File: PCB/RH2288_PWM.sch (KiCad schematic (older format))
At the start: 10 parts, among them J1 Conn_01x01, J2 AVR_ICSP, J3 Conn_FANs, J4 Conn_RH2288_V2, J5 UART, U1 78L05_SOT23, U2 ATmega328P-MMH

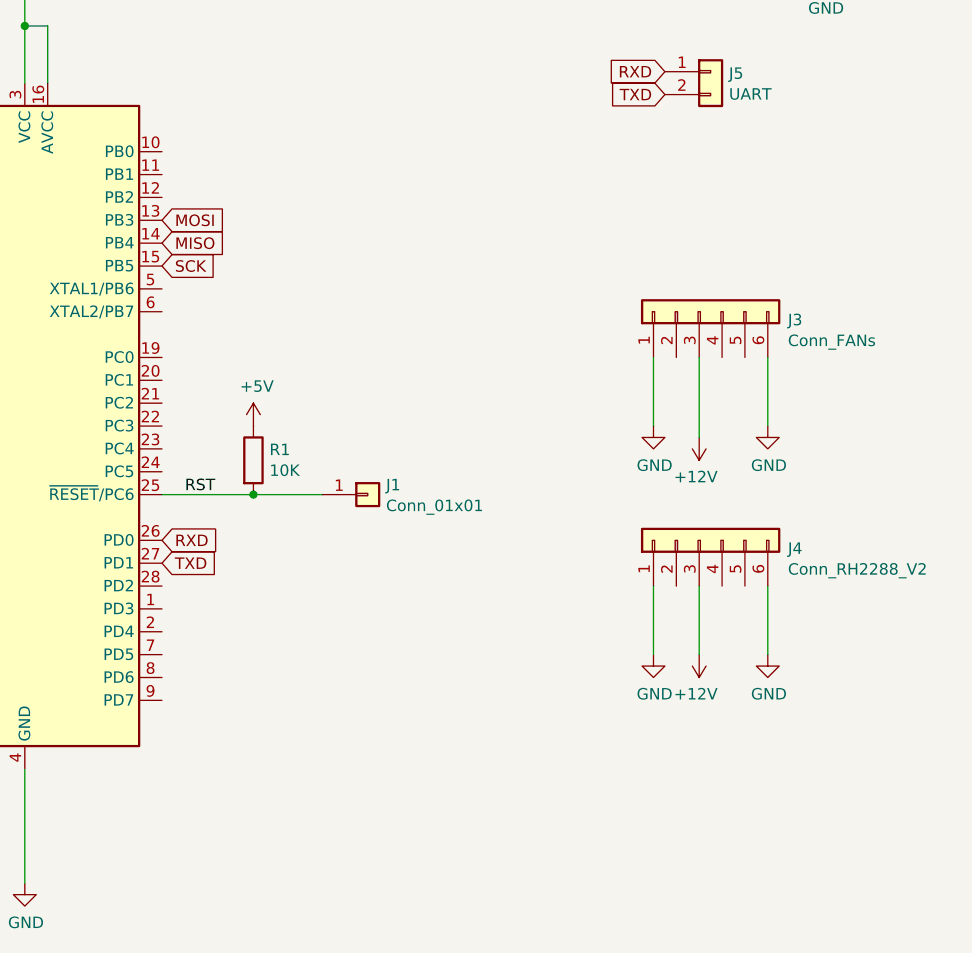
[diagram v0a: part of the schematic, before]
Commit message: PCB finished
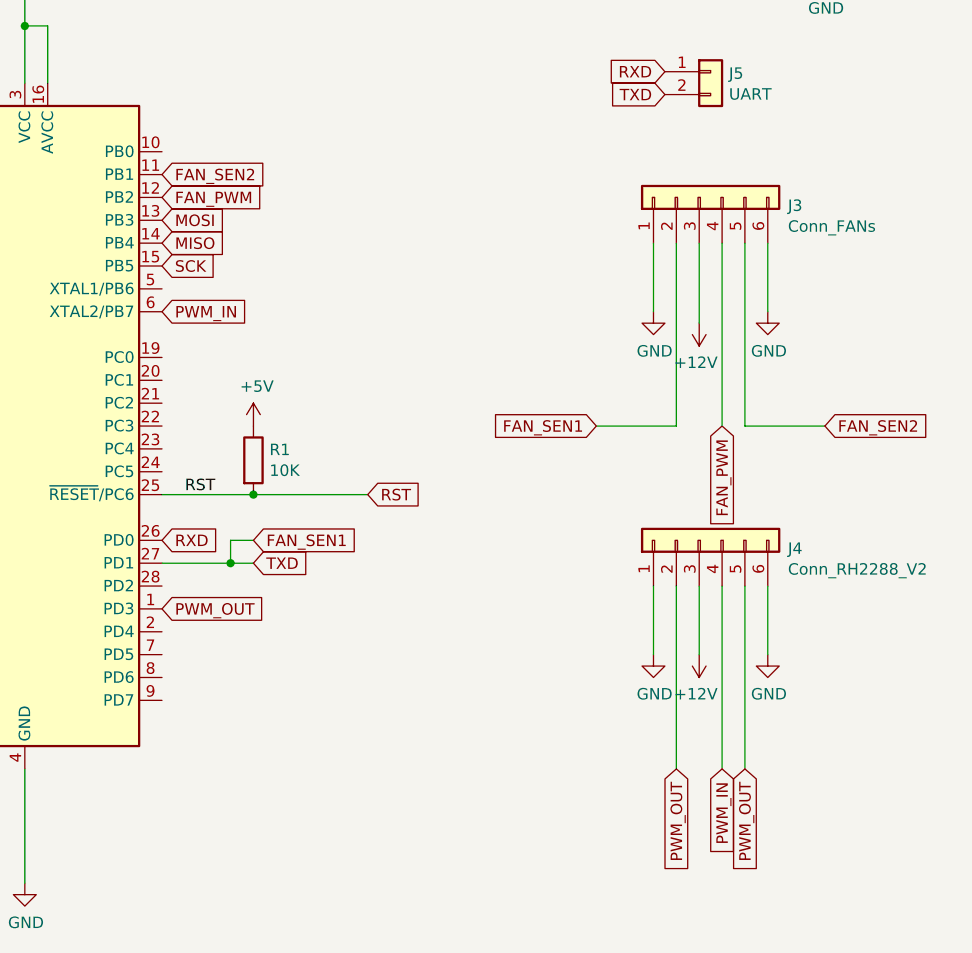
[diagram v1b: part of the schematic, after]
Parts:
- removed J1: Conn_01x01, Connector_PinHeader_2.54mm:PinHeader_1x01_P2.54mm_Vertical, symbol Connector_Generic:Conn_01x01
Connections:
- net TXD is gone; now on net FAN_SEN1: J5.2 (Pin_2), U2.27 (PD1)
- net PWM_OUT: now reaches U2.1 (PD3)
- net PWM_OUT: now also J4.2 (Pin_2), J4.5 (Pin_5)
- net FAN_SEN2: now reaches U2.11 (PB1)
- net FAN_SEN2: now also J3.5 (Pin_5)
- net FAN_PWM: now reaches U2.12 (PB2)
- net FAN_PWM: now also J3.4 (Pin_4)
- net PWM_IN: now reaches U2.6 (XTAL2/PB7)
- net PWM_IN: now also J4.4 (Pin_4)
- net FAN_SEN1: now reaches J3.2 (Pin_2)
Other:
- moved on the sheet: J3
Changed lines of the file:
@@
 Text GLabel 6100 3300 2    50   Input ~ 0
 SCK
-Text GLabel 6100 4600 2    50   Input ~ 0
+Text GLabel 6500 4600 2    50   Input ~ 0
 TXD
 Text GLabel 6100 4500 2    50   Input ~ 0
@@
 Wire Wire Line
 	6500 4300 6100 4300
-$Comp
-L Connector_Generic:Conn_01x01 J1
-U 1 1 5E729BF9
-P 7000 4300
-F 0 "J1" H 7080 4342 50  0000 L CNN
-F 1 "Conn_01x01" H 7080 4251 50  0000 L CNN
-F 2 "Connector_PinHeader_2.54mm:PinHeader_1x01_P2.54mm_Vertical" H 7000 4300 50  0001 C CNN
-F 3 "~" H 7000 4300 50  0001 C CNN
-	1    7000 4300
-	1    0    0    -1
-$EndComp
-Wire Wire Line
-	6800 4300 6500 4300
-Connection ~ 6500 4300
 Text Label 6200 4300 0    50   ~ 0
 RST
@@
 L Connector_Generic:Conn_01x06 J3
 U 1 1 5E72F58C
-P 8450 3500
-F 0 "J3" V 8414 3112 50  0000 R CNN
-F 1 "Conn_FANs" V 8323 3112 50  0000 R CNN
-F 2 "Connector_PinHeader_2.54mm:PinHeader_1x06_P2.54mm_Horizontal" H 8450 3500 50  0001 C CNN
-F 3 "~" H 8450 3500 50  0001 C CNN
-	1    8450 3500
+P 8450 3000
+F 0 "J3" V 8414 2612 50  0000 R CNN
+F 1 "Conn_FANs" V 8323 2612 50  0000 R CNN
+F 2 "Connector_PinHeader_2.54mm:PinHeader_1x06_P2.54mm_Horizontal" H 8450 3000 50  0001 C CNN
+F 3 "~" H 8450 3000 50  0001 C CNN
+	1    8450 3000
 	0    -1   -1   0
 $EndComp
@@
 L power:GND #PWR0112
 U 1 1 5E730F06
-P 8250 4000
-F 0 "#PWR0112" H 8250 3750 50  0001 C CNN
-F 1 "GND" H 8255 3827 50  0000 C CNN
-F 2 "" H 8250 4000 50  0001 C CNN
-F 3 "" H 8250 4000 50  0001 C CNN
-	1    8250 4000
+P 8250 3500
+F 0 "#PWR0112" H 8250 3250 50  0001 C CNN
+F 1 "GND" H 8255 3327 50  0000 C CNN
+F 2 "" H 8250 3500 50  0001 C CNN
+F 3 "" H 8250 3500 50  0001 C CNN
+	1    8250 3500
 	1    0    0    -1
 $EndComp
@@
 L power:GND #PWR0113
 U 1 1 5E731799
-P 8750 4000
-F 0 "#PWR0113" H 8750 3750 50  0001 C CNN
-F 1 "GND" H 8755 3827 50  0000 C CNN
-F 2 "" H 8750 4000 50  0001 C CNN
-F 3 "" H 8750 4000 50  0001 C CNN
-	1    8750 4000
+P 8750 3500
+F 0 "#PWR0113" H 8750 3250 50  0001 C CNN
+F 1 "GND" H 8755 3327 50  0000 C CNN
+F 2 "" H 8750 3500 50  0001 C CNN
+F 3 "" H 8750 3500 50  0001 C CNN
+	1    8750 3500
 	1    0    0    -1
 $EndComp
@@
 	8250 5000 8250 4700
 Wire Wire Line
-	8250 4000 8250 3700
-Wire Wire Line
-	8750 3700 8750 4000
+	8250 3500 8250 3200
+Wire Wire Line
+	8750 3200 8750 3500
 $Comp
 L power:+12V #PWR0116
@@
 L power:+12V #PWR0117
 U 1 1 5E734C90
-P 8450 4050
-F 0 "#PWR0117" H 8450 3900 50  0001 C CNN
-F 1 "+12V" H 8465 4223 50  0000 C CNN
-F 2 "" H 8450 4050 50  0001 C CNN
-F 3 "" H 8450 4050 50  0001 C CNN
-	1    8450 4050
+P 8450 3550
+F 0 "#PWR0117" H 8450 3400 50  0001 C CNN
+F 1 "+12V" H 8465 3723 50  0000 C CNN
+F 2 "" H 8450 3550 50  0001 C CNN
+F 3 "" H 8450 3550 50  0001 C CNN
+	1    8450 3550
 	-1   0    0    1
 $EndComp
 Wire Wire Line
-	8450 4050 8450 3700
+	8450 3550 8450 3200
 Wire Wire Line
 	8450 4700 8450 5000
@@
 	1    0    0    -1
 $EndComp
+Text GLabel 8550 5500 3    50   Input ~ 0
+PWM_IN
+Wire Wire Line
+	8550 5500 8550 4700
+Text GLabel 8350 5500 3    50   Input ~ 0
+PWM_OUT
+Text GLabel 8650 5500 3    50   Input ~ 0
+PWM_OUT
+Wire Wire Line
+	8650 5500 8650 4700
+Wire Wire Line
+	8350 5500 8350 4700
+Text GLabel 8550 4000 3    50   Input ~ 0
+FAN_PWM
+Text GLabel 8000 4000 0    50   Input ~ 0
+FAN_SEN1
+Text GLabel 9000 4000 2    50   Input ~ 0
+FAN_SEN2
+Wire Wire Line
+	8000 4000 8350 4000
+Wire Wire Line
+	8350 4000 8350 3200
+Wire Wire Line
+	8550 3200 8550 4000
+Wire Wire Line
+	8650 3200 8650 4000
+Wire Wire Line
+	8650 4000 9000 4000
+Text GLabel 6100 3000 2    50   Input ~ 0
+FAN_PWM
+Text GLabel 6100 4800 2    50   Input ~ 0
+PWM_OUT
+Text GLabel 6100 3500 2    50   Input ~ 0
+PWM_IN
+Text GLabel 6100 2900 2    50   Input ~ 0
+FAN_SEN2
+Text GLabel 6500 4500 2    50   Input ~ 0
+FAN_SEN1
+Wire Wire Line
+	6500 4600 6400 4600
+Wire Wire Line
+	6500 4500 6400 4500
+Wire Wire Line
+	6400 4500 6400 4600
+Connection ~ 6400 4600
+Wire Wire Line
+	6400 4600 6100 4600
+Text GLabel 7000 4300 2    50   Input ~ 0
+RST
+Wire Wire Line
+	7000 4300 6500 4300
+Connection ~ 6500 4300
 $EndSCHEMATC
